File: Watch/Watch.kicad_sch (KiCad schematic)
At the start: 0 parts

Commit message: schematics
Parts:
- added A1: RaspberryPi_Pico, Module:RaspberryPi_Pico_Common_Unspecified, symbol MCU_Module:RaspberryPi_Pico
- added C1: C_Small, Package_SO:SOIC-8_3.9x4.9mm_P1.27mm, symbol Device:C_Small
- added J1: Conn_01x11_Pin, symbol Connector:Conn_01x11_Pin
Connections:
- new net +3V3: A1.36 (3V3), J1.10 (Pin_10), J1.11 (Pin_11)
- new net CHIP SELECT: A1.2 (GPIO1), J1.5 (Pin_5)
- new net CS: A1.22 (GPIO17)
- new net DATA: A1.5 (GPIO3), J1.3 (Pin_3)
- new net GND: A1.13 (GND), A1.18 (GND), A1.23 (GND), A1.28 (GND), A1.3 (GND), A1.33 (AGND), A1.38 (GND), A1.8 (GND), J1.4 (Pin_4), J1.9 (Pin_9)
- new net MISO: A1.26 (GPIO20), J1.7 (Pin_7)
- new net MOSI: A1.25 (GPIO19), J1.6 (Pin_6)
- new net OFFLINE: A1.4 (GPIO2), J1.2 (Pin_2)
- new net SCK: A1.24 (GPIO18), J1.8 (Pin_8)
- new net TFT_BL: A1.1 (GPIO0), J1.1 (Pin_1)
- no-connect marks 0 -> 20

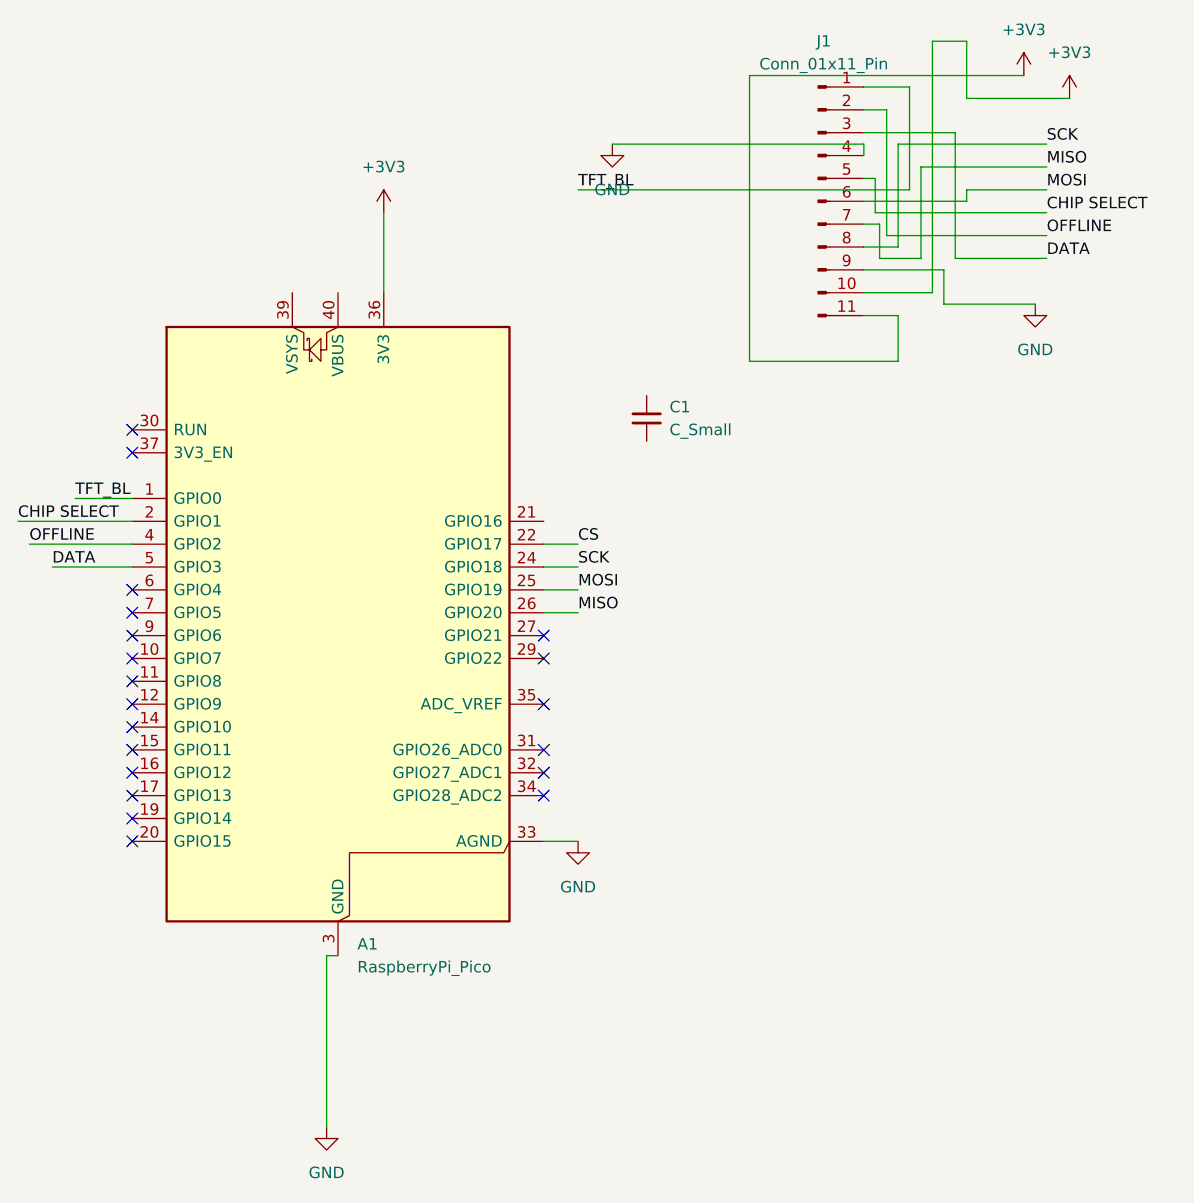
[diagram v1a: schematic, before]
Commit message: FINISHED
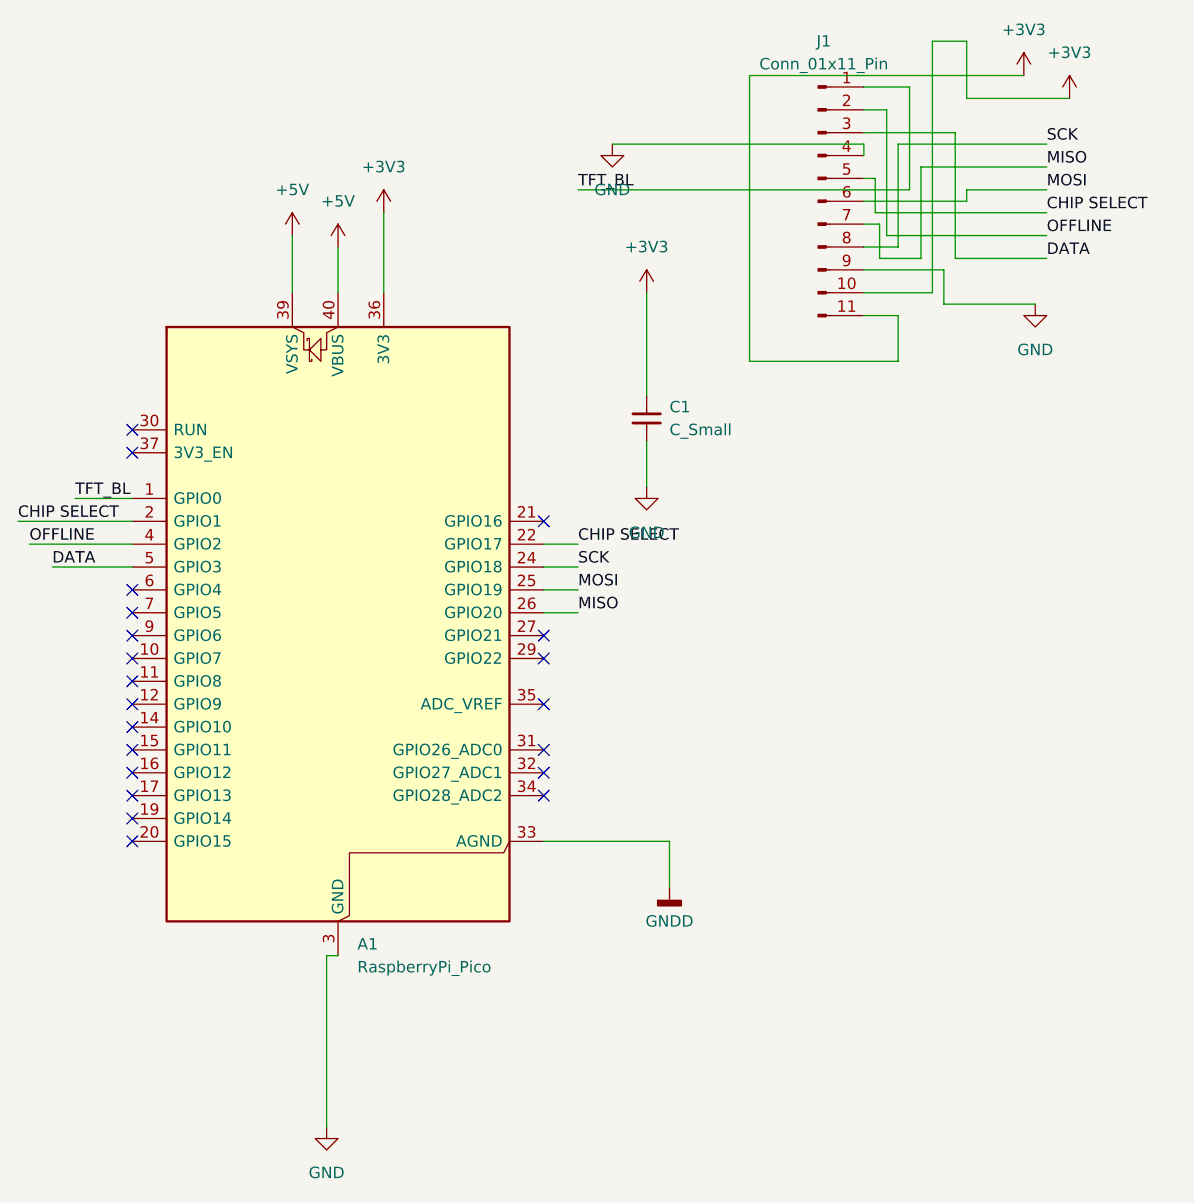
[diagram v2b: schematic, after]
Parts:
- J1: footprint (none) -> Connector_PinHeader_2.54mm:PinHeader_1x11_P2.54mm_Horizontal
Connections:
- net CS is gone; now on net CHIP SELECT: A1.22 (GPIO17)
- net +3V3: now also C1.1
- net GND: now also C1.2; no longer A1.33 (AGND)
- net +5V: now reaches A1.39 (VSYS)
- net +5V: now also A1.40 (VBUS)
- new net GNDD: A1.33 (AGND)
- no-connect marks 20 -> 21
